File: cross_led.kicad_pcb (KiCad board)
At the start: 2 copper layers, 40 x 40 mm, 25 parts, among them J201 Conn_01x03_Pin, J202 Conn_01x03_Pin, J203 Conn_01x03_Pin, J204 Conn_01x03_Pin, Q201 NMOS

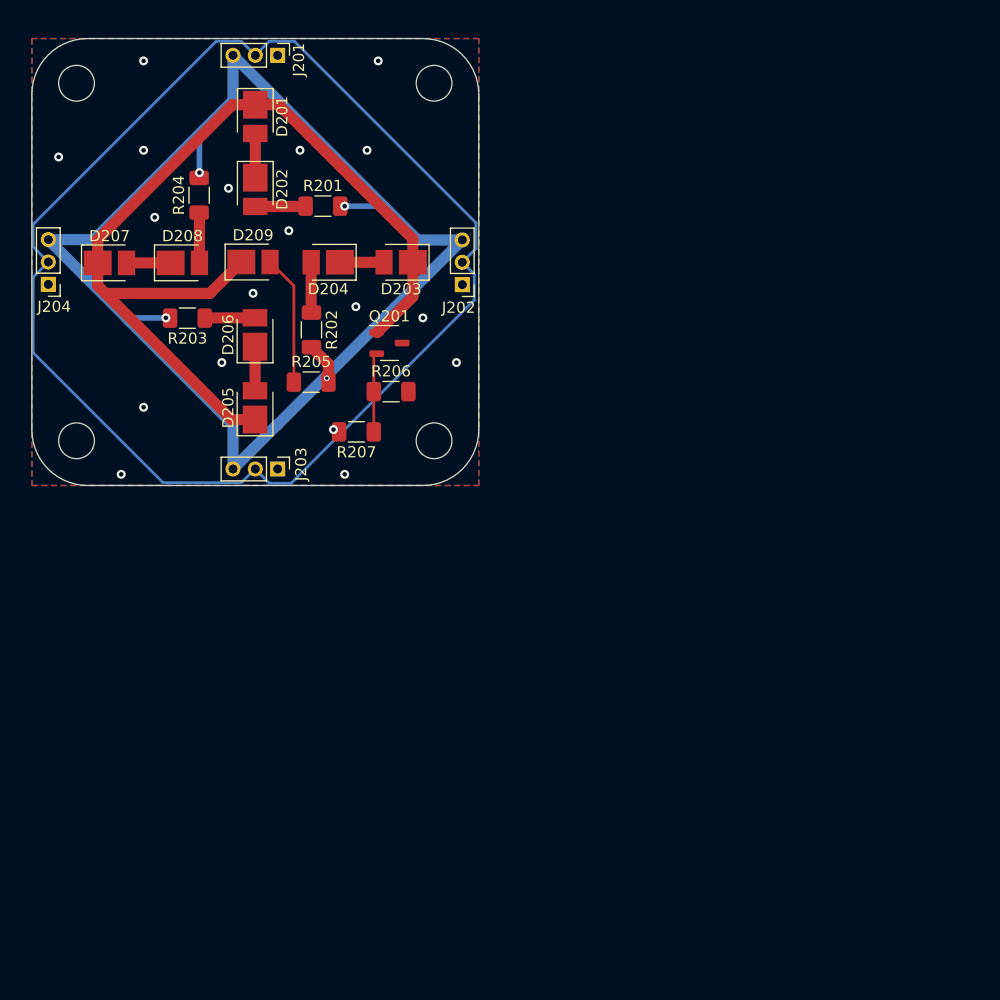
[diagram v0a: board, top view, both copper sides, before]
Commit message: gerber
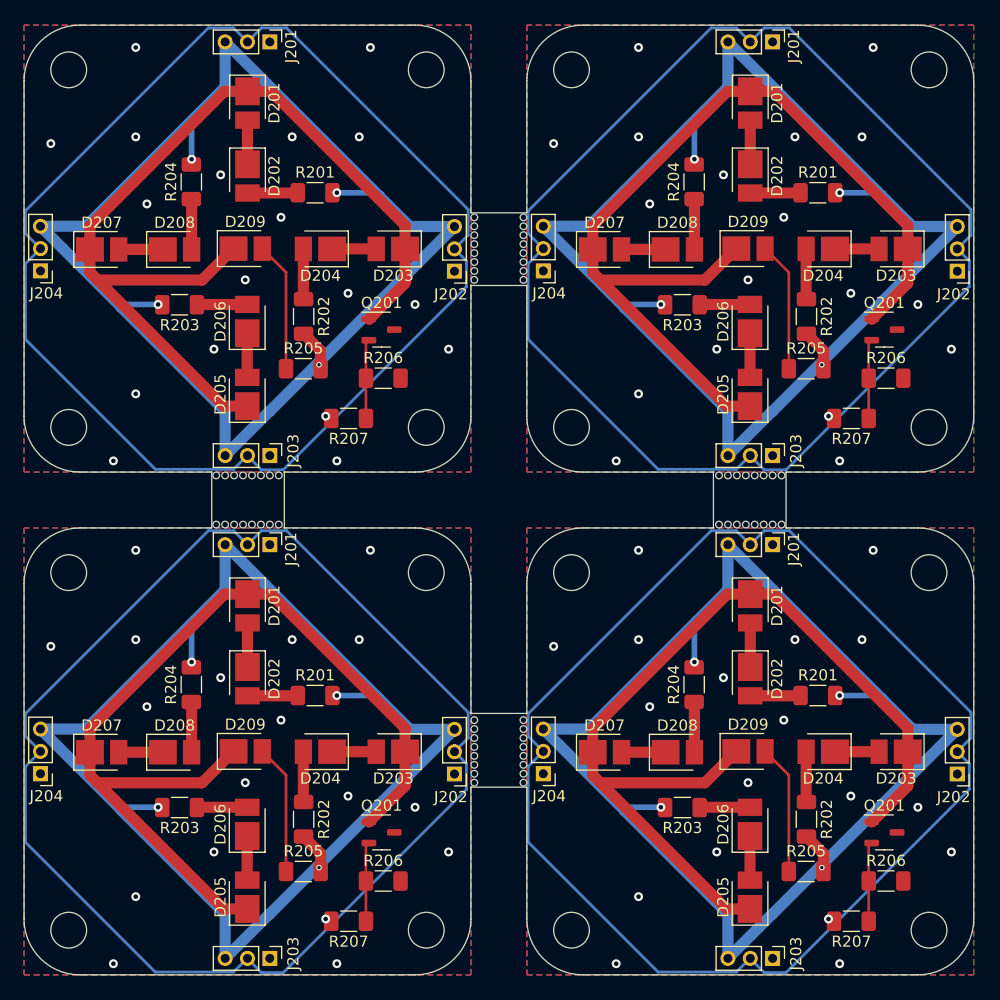
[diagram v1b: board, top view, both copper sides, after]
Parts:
- removed the D201 at (120.0, 57.0)
- removed the D202 at (120.0, 63.5)
- removed the D203 at (133.1, 70.0)
- removed the D204 at (126.5, 70.0)
- removed the D205 at (120.0, 83.0)
- removed the D206 at (120.0, 76.5)
- removed the D207 at (107.0, 70.1)
- removed the D208 at (113.5, 70.1)
- removed the D209 at (119.8, 70.0)
- removed the J201 at (122.0, 51.5)
- removed the J202 at (138.5, 72.0)
- removed the J203 at (122.0, 88.5)
- removed the J204 at (101.5, 72.0)
- removed the Q201 at (132.0, 77.2)
- removed the R201 at (126.0, 65.0)
- removed the R202 at (125.0, 76.1)
- removed the R203 at (113.9, 75.0)
- removed the R204 at (115.0, 64.0)
- removed the R205 at (125.0, 80.8)
- removed the R206 at (132.2, 81.6)
- removed the R207 at (129.1, 85.2)
- removed the REF** at (136.0, 54.0)
- removed the REF** at (104.0, 54.0)
- removed the REF** at (136.0, 86.0)
- removed the REF** at (104.0, 86.0)
- added D201: LED, LED_SMD:LED_PLCC_2835_Handsoldering, F.Cu at (164.3, 100.8)
- added D201: LED, LED_SMD:LED_PLCC_2835_Handsoldering, F.Cu at (164.3, 55.8)
- added D201: LED, LED_SMD:LED_PLCC_2835_Handsoldering, F.Cu at (119.3, 100.8)
- added D201: LED, LED_SMD:LED_PLCC_2835_Handsoldering, F.Cu at (119.3, 55.8)
- added D202: LED, LED_SMD:LED_PLCC_2835_Handsoldering, F.Cu at (164.3, 107.3)
- added D202: LED, LED_SMD:LED_PLCC_2835_Handsoldering, F.Cu at (164.3, 62.3)
- added D202: LED, LED_SMD:LED_PLCC_2835_Handsoldering, F.Cu at (119.3, 107.3)
- added D202: LED, LED_SMD:LED_PLCC_2835_Handsoldering, F.Cu at (119.3, 62.3)
- added D203: LED, LED_SMD:LED_PLCC_2835_Handsoldering, F.Cu at (177.3, 113.8)
- added D203: LED, LED_SMD:LED_PLCC_2835_Handsoldering, F.Cu at (177.3, 68.8)
- added D203: LED, LED_SMD:LED_PLCC_2835_Handsoldering, F.Cu at (132.3, 113.8)
- added D203: LED, LED_SMD:LED_PLCC_2835_Handsoldering, F.Cu at (132.3, 68.8)
- added D204: LED, LED_SMD:LED_PLCC_2835_Handsoldering, F.Cu at (170.8, 113.8)
- added D204: LED, LED_SMD:LED_PLCC_2835_Handsoldering, F.Cu at (170.8, 68.8)
- added D204: LED, LED_SMD:LED_PLCC_2835_Handsoldering, F.Cu at (125.8, 68.8)
- added D204: LED, LED_SMD:LED_PLCC_2835_Handsoldering, F.Cu at (125.8, 113.8)
- added D205: LED, LED_SMD:LED_PLCC_2835_Handsoldering, F.Cu at (119.3, 81.8)
- added D205: LED, LED_SMD:LED_PLCC_2835_Handsoldering, F.Cu at (164.3, 81.8)
- added D205: LED, LED_SMD:LED_PLCC_2835_Handsoldering, F.Cu at (164.3, 126.8)
- added D205: LED, LED_SMD:LED_PLCC_2835_Handsoldering, F.Cu at (119.3, 126.8)
- added D206: LED, LED_SMD:LED_PLCC_2835_Handsoldering, F.Cu at (119.3, 75.3)
- added D206: LED, LED_SMD:LED_PLCC_2835_Handsoldering, F.Cu at (164.3, 75.3)
- added D206: LED, LED_SMD:LED_PLCC_2835_Handsoldering, F.Cu at (119.3, 120.3)
- added D206: LED, LED_SMD:LED_PLCC_2835_Handsoldering, F.Cu at (164.3, 120.3)
- added D207: LED, LED_SMD:LED_PLCC_2835_Handsoldering, F.Cu at (106.2, 113.9)
- added D207: LED, LED_SMD:LED_PLCC_2835_Handsoldering, F.Cu at (151.2, 68.9)
- added D207: LED, LED_SMD:LED_PLCC_2835_Handsoldering, F.Cu at (151.2, 113.9)
- added D207: LED, LED_SMD:LED_PLCC_2835_Handsoldering, F.Cu at (106.2, 68.9)
- added D208: LED, LED_SMD:LED_PLCC_2835_Handsoldering, F.Cu at (112.8, 113.9)
- added D208: LED, LED_SMD:LED_PLCC_2835_Handsoldering, F.Cu at (157.8, 68.9)
- added D208: LED, LED_SMD:LED_PLCC_2835_Handsoldering, F.Cu at (112.8, 68.9)
- added D208: LED, LED_SMD:LED_PLCC_2835_Handsoldering, F.Cu at (157.8, 113.9)
- added D209: LED, LED_SMD:LED_PLCC_2835_Handsoldering, F.Cu at (164.1, 113.8)
- added D209: LED, LED_SMD:LED_PLCC_2835_Handsoldering, F.Cu at (119.1, 68.8)
- added D209: LED, LED_SMD:LED_PLCC_2835_Handsoldering, F.Cu at (119.1, 113.8)
- added D209: LED, LED_SMD:LED_PLCC_2835_Handsoldering, F.Cu at (164.1, 68.8)
- added J201: Conn_01x03_Pin, Connector_PinHeader_2.00mm:PinHeader_1x03_P2.00mm_Vertical, F.Cu at (121.3, 50.3)
- added J201: Conn_01x03_Pin, Connector_PinHeader_2.00mm:PinHeader_1x03_P2.00mm_Vertical, F.Cu at (166.3, 95.3)
- added J201: Conn_01x03_Pin, Connector_PinHeader_2.00mm:PinHeader_1x03_P2.00mm_Vertical, F.Cu at (121.3, 95.3)
- added J201: Conn_01x03_Pin, Connector_PinHeader_2.00mm:PinHeader_1x03_P2.00mm_Vertical, F.Cu at (166.3, 50.3)
- added J202: Conn_01x03_Pin, Connector_PinHeader_2.00mm:PinHeader_1x03_P2.00mm_Vertical, F.Cu at (182.8, 70.8)
- added J202: Conn_01x03_Pin, Connector_PinHeader_2.00mm:PinHeader_1x03_P2.00mm_Vertical, F.Cu at (182.8, 115.8)
- added J202: Conn_01x03_Pin, Connector_PinHeader_2.00mm:PinHeader_1x03_P2.00mm_Vertical, F.Cu at (137.8, 115.8)
- added J202: Conn_01x03_Pin, Connector_PinHeader_2.00mm:PinHeader_1x03_P2.00mm_Vertical, F.Cu at (137.8, 70.8)
- added J203: Conn_01x03_Pin, Connector_PinHeader_2.00mm:PinHeader_1x03_P2.00mm_Vertical, F.Cu at (121.3, 132.3)
- added J203: Conn_01x03_Pin, Connector_PinHeader_2.00mm:PinHeader_1x03_P2.00mm_Vertical, F.Cu at (166.3, 87.3)
- added J203: Conn_01x03_Pin, Connector_PinHeader_2.00mm:PinHeader_1x03_P2.00mm_Vertical, F.Cu at (121.3, 87.3)
- added J203: Conn_01x03_Pin, Connector_PinHeader_2.00mm:PinHeader_1x03_P2.00mm_Vertical, F.Cu at (166.3, 132.3)
- added J204: Conn_01x03_Pin, Connector_PinHeader_2.00mm:PinHeader_1x03_P2.00mm_Vertical, F.Cu at (145.8, 70.8)
- added J204: Conn_01x03_Pin, Connector_PinHeader_2.00mm:PinHeader_1x03_P2.00mm_Vertical, F.Cu at (145.8, 115.8)
- added J204: Conn_01x03_Pin, Connector_PinHeader_2.00mm:PinHeader_1x03_P2.00mm_Vertical, F.Cu at (100.8, 115.8)
- added J204: Conn_01x03_Pin, Connector_PinHeader_2.00mm:PinHeader_1x03_P2.00mm_Vertical, F.Cu at (100.8, 70.8)
- added Q201: NMOS, Package_TO_SOT_SMD:SOT-23-3, F.Cu at (131.3, 121.0)
- added Q201: NMOS, Package_TO_SOT_SMD:SOT-23-3, F.Cu at (131.3, 76.0)
- added Q201: NMOS, Package_TO_SOT_SMD:SOT-23-3, F.Cu at (176.3, 76.0)
- added Q201: NMOS, Package_TO_SOT_SMD:SOT-23-3, F.Cu at (176.3, 121.0)
- added R201: 47Ω, Resistor_SMD:R_1206_3216Metric_Pad1.30x1.75mm_HandSolder, F.Cu at (125.3, 63.8)
- added R201: 47Ω, Resistor_SMD:R_1206_3216Metric_Pad1.30x1.75mm_HandSolder, F.Cu at (170.3, 108.8)
- added R201: 47Ω, Resistor_SMD:R_1206_3216Metric_Pad1.30x1.75mm_HandSolder, F.Cu at (125.3, 108.8)
- added R201: 47Ω, Resistor_SMD:R_1206_3216Metric_Pad1.30x1.75mm_HandSolder, F.Cu at (170.3, 63.8)
- added R202: 47Ω, Resistor_SMD:R_1206_3216Metric_Pad1.30x1.75mm_HandSolder, F.Cu at (124.3, 119.9)
- added R202: 47Ω, Resistor_SMD:R_1206_3216Metric_Pad1.30x1.75mm_HandSolder, F.Cu at (169.3, 119.9)
- added R202: 47Ω, Resistor_SMD:R_1206_3216Metric_Pad1.30x1.75mm_HandSolder, F.Cu at (124.3, 74.9)
- added R202: 47Ω, Resistor_SMD:R_1206_3216Metric_Pad1.30x1.75mm_HandSolder, F.Cu at (169.3, 74.9)
- added R203: 47Ω, Resistor_SMD:R_1206_3216Metric_Pad1.30x1.75mm_HandSolder, F.Cu at (158.2, 118.8)
- added R203: 47Ω, Resistor_SMD:R_1206_3216Metric_Pad1.30x1.75mm_HandSolder, F.Cu at (113.2, 118.8)
- added R203: 47Ω, Resistor_SMD:R_1206_3216Metric_Pad1.30x1.75mm_HandSolder, F.Cu at (158.2, 73.8)
- added R203: 47Ω, Resistor_SMD:R_1206_3216Metric_Pad1.30x1.75mm_HandSolder, F.Cu at (113.2, 73.8)
- added R204: 47Ω, Resistor_SMD:R_1206_3216Metric_Pad1.30x1.75mm_HandSolder, F.Cu at (114.3, 107.8)
- added R204: 47Ω, Resistor_SMD:R_1206_3216Metric_Pad1.30x1.75mm_HandSolder, F.Cu at (114.3, 62.8)
- added R204: 47Ω, Resistor_SMD:R_1206_3216Metric_Pad1.30x1.75mm_HandSolder, F.Cu at (159.3, 107.8)
- added R204: 47Ω, Resistor_SMD:R_1206_3216Metric_Pad1.30x1.75mm_HandSolder, F.Cu at (159.3, 62.8)
- added R205: 47Ω, Resistor_SMD:R_1206_3216Metric_Pad1.30x1.75mm_HandSolder, F.Cu at (169.3, 124.5)
- added R205: 47Ω, Resistor_SMD:R_1206_3216Metric_Pad1.30x1.75mm_HandSolder, F.Cu at (169.3, 79.5)
- added R205: 47Ω, Resistor_SMD:R_1206_3216Metric_Pad1.30x1.75mm_HandSolder, F.Cu at (124.3, 124.5)
- added R205: 47Ω, Resistor_SMD:R_1206_3216Metric_Pad1.30x1.75mm_HandSolder, F.Cu at (124.3, 79.5)
- added R206: 10kΩ, Resistor_SMD:R_1206_3216Metric_Pad1.30x1.75mm_HandSolder, F.Cu at (176.4, 80.4)
- added R206: 10kΩ, Resistor_SMD:R_1206_3216Metric_Pad1.30x1.75mm_HandSolder, F.Cu at (131.4, 125.4)
- added R206: 10kΩ, Resistor_SMD:R_1206_3216Metric_Pad1.30x1.75mm_HandSolder, F.Cu at (176.4, 125.4)
- added R206: 10kΩ, Resistor_SMD:R_1206_3216Metric_Pad1.30x1.75mm_HandSolder, F.Cu at (131.4, 80.4)
- added R207: 100Ω, Resistor_SMD:R_1206_3216Metric_Pad1.30x1.75mm_HandSolder, F.Cu at (128.3, 129.0)
- added R207: 100Ω, Resistor_SMD:R_1206_3216Metric_Pad1.30x1.75mm_HandSolder, F.Cu at (173.3, 129.0)
- added R207: 100Ω, Resistor_SMD:R_1206_3216Metric_Pad1.30x1.75mm_HandSolder, F.Cu at (128.3, 84.0)
- added R207: 100Ω, Resistor_SMD:R_1206_3216Metric_Pad1.30x1.75mm_HandSolder, F.Cu at (173.3, 84.0)
- added REF**: MountingHole_3.2mm_M3, MountingHole:MountingHole_3.2mm_M3, F.Cu at (103.3, 84.8)
- added REF**: MountingHole_3.2mm_M3, MountingHole:MountingHole_3.2mm_M3, F.Cu at (148.3, 52.8)
- added REF**: MountingHole_3.2mm_M3, MountingHole:MountingHole_3.2mm_M3, F.Cu at (148.3, 97.8)
- added REF**: MountingHole_3.2mm_M3, MountingHole:MountingHole_3.2mm_M3, F.Cu at (148.3, 84.8)
- added REF**: MountingHole_3.2mm_M3, MountingHole:MountingHole_3.2mm_M3, F.Cu at (103.3, 52.8)
- added REF**: MountingHole_3.2mm_M3, MountingHole:MountingHole_3.2mm_M3, F.Cu at (135.3, 129.8)
- added REF**: MountingHole_3.2mm_M3, MountingHole:MountingHole_3.2mm_M3, F.Cu at (103.3, 97.8)
- added REF**: MountingHole_3.2mm_M3, MountingHole:MountingHole_3.2mm_M3, F.Cu at (180.3, 129.8)
- added REF**: MountingHole_3.2mm_M3, MountingHole:MountingHole_3.2mm_M3, F.Cu at (180.3, 84.8)
- added REF**: bridge, LIB:bridge, F.Cu at (167.5, 93.8)
- added REF**: MountingHole_3.2mm_M3, MountingHole:MountingHole_3.2mm_M3, F.Cu at (180.3, 52.8)
- added REF**: MountingHole_3.2mm_M3, MountingHole:MountingHole_3.2mm_M3, F.Cu at (180.3, 97.8)
- added REF**: bridge, LIB:bridge, F.Cu at (144.3, 65.6)
- added REF**: MountingHole_3.2mm_M3, MountingHole:MountingHole_3.2mm_M3, F.Cu at (135.3, 97.8)
- added REF**: MountingHole_3.2mm_M3, MountingHole:MountingHole_3.2mm_M3, F.Cu at (135.3, 52.8)
- added REF**: bridge, LIB:bridge, F.Cu at (116.1, 88.8)
- added REF**: MountingHole_3.2mm_M3, MountingHole:MountingHole_3.2mm_M3, F.Cu at (148.3, 129.8)
- added REF**: MountingHole_3.2mm_M3, MountingHole:MountingHole_3.2mm_M3, F.Cu at (135.3, 84.8)
- added REF**: bridge, LIB:bridge, F.Cu at (139.3, 117.0)
- added REF**: MountingHole_3.2mm_M3, MountingHole:MountingHole_3.2mm_M3, F.Cu at (103.3, 129.8)
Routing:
- net /cross_led/LED_IN: track 127.5 -> 509.9 mm, vias 1 -> 4
- net +5V: track 124.5 -> 497.8 mm, vias 4 -> 16
- net Net-(D201-K): track 84.4 -> 337.7 mm
- net Net-(D209-A): track 11.6 -> 46.5 mm
- net Net-(Q201-G): track 7.11 -> 28.4 mm
- net Net-(D206-A): track 4.51 -> 18.0 mm
- net Net-(D202-A): track 4.51 -> 18.0 mm
- net Net-(D208-A): track 4.51 -> 18.0 mm
- net Net-(D204-A): track 4.51 -> 18.0 mm
- net Net-(D205-A): track 3.95 -> 15.8 mm
- net Net-(D201-A): track 3.95 -> 15.8 mm
- net Net-(D207-A): track 3.95 -> 15.8 mm
- net Net-(D203-A): track 3.95 -> 15.8 mm
- net GND: vias 17 -> 68
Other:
- board size 40 x 40 mm -> 85 x 85 mm
